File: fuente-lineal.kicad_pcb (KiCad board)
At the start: 2 copper layers, 100 x 74 mm, 34 parts, among them J1 Conn_01x03, J2 Conn_01x03, J3 Conn_01x01, J4 Conn_01x01, J5 Conn_01x01, J6 Conn_01x01, J7 Conn_01x01, J8 Conn_01x01, J9 Conn_01x02, U1 LM7805_TO220

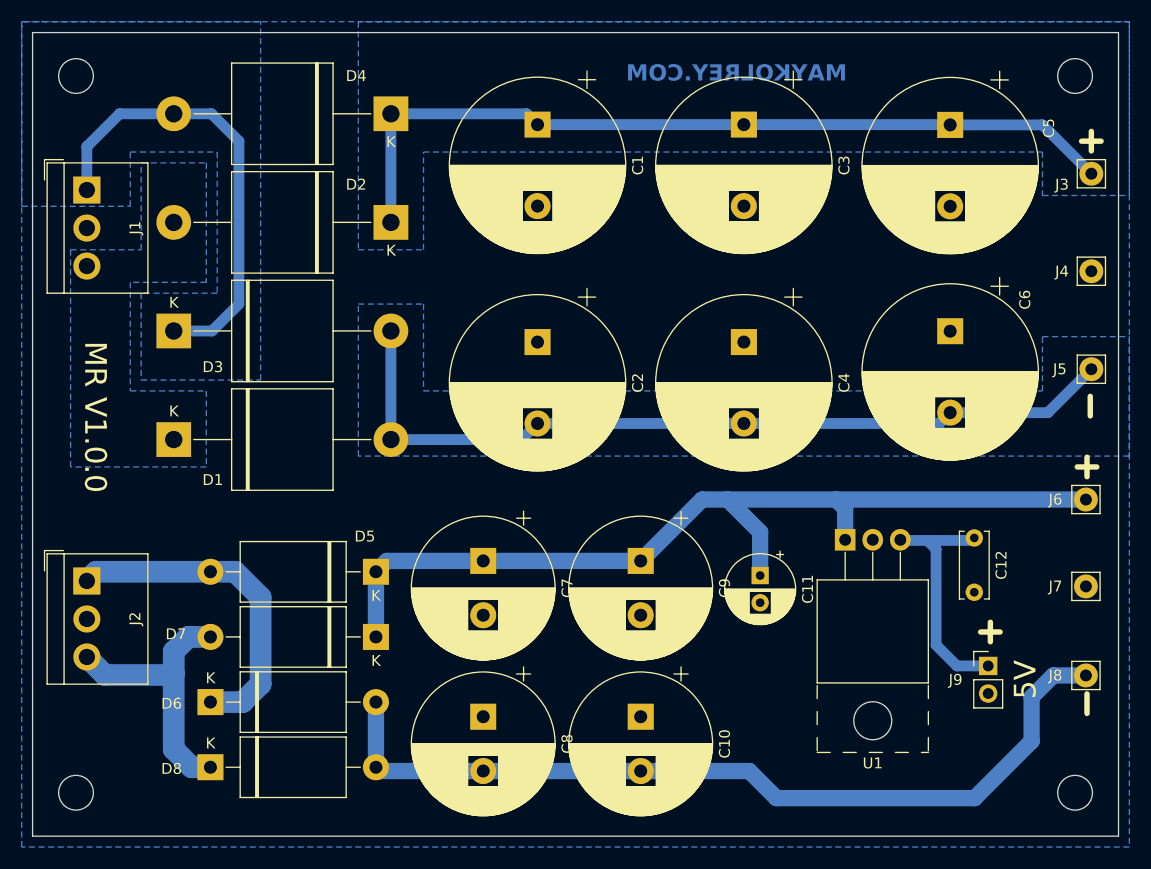
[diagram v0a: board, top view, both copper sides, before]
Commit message: completando version v1.1.0
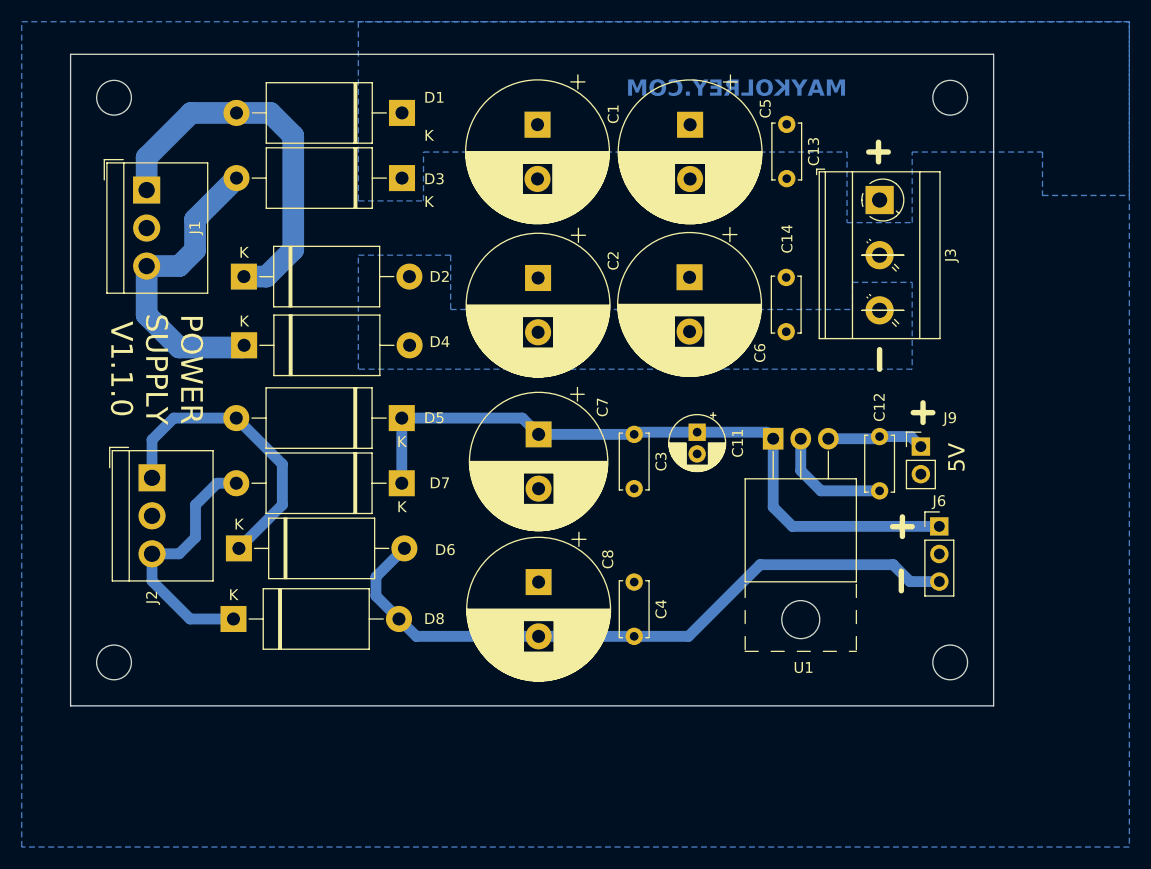
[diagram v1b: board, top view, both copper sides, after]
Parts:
- removed C10, C9: 2200uF, Capacitor_THT:CP_Radial_D13.0mm_P5.00mm
- removed J4, J5, J7, J8: Conn_01x01, Connector_Pin:Pin_D1.1mm_L8.5mm_W2.5mm_FlatFork
- added C13: 100nF, Capacitor_THT:C_Disc_D5.0mm_W2.5mm_P5.00mm, F.Cu at (164.4, 71.5)
- added C14: 100nF, Capacitor_THT:C_Disc_D5.0mm_W2.5mm_P5.00mm, F.Cu at (164.4, 85.5)
- C1, C2, C5, C6: footprint Capacitor_THT:CP_Radial_D16.0mm_P7.50mm -> Capacitor_THT:CP_Radial_D13.0mm_P5.00mm
- C11: value 0.33u -> 2.2uF; footprint Capacitor_THT:CP_Radial_D6.3mm_P2.50mm -> Capacitor_THT:CP_Radial_D5.0mm_P2.00mm
- C12: value C -> 100nF; footprint Capacitor_THT:C_Disc_D6.0mm_W2.5mm_P5.00mm -> Capacitor_THT:C_Disc_D5.0mm_W2.5mm_P5.00mm
- C3, C4: value 2200uF -> 100nF; footprint Capacitor_THT:CP_Radial_D16.0mm_P7.50mm -> Capacitor_THT:C_Disc_D5.0mm_W2.5mm_P5.00mm
- C7: footprint Capacitor_THT:CP_Radial_D13.0mm_P5.00mm -> Capacitor_THT:CP_Radial_D12.5mm_P5.00mm
- D1, D2, D3, D4: value 6A10 -> 1N5404; footprint Diode_THT:D_P600_R-6_P20.00mm_Horizontal -> Diode_THT:D_DO-27_P15.24mm_Horizontal
- J3: value Conn_01x01 -> Conn_01x03; footprint Connector_Pin:Pin_D1.1mm_L8.5mm_W2.5mm_FlatFork -> TerminalBlock_MetzConnect:TerminalBlock_MetzConnect_Type073_RT02603HBLU_1x03_P5.08mm_Horizontal
- J6: value Conn_01x01 -> Conn_01x03; footprint Connector_Pin:Pin_D1.1mm_L8.5mm_W2.5mm_FlatFork -> Connector_PinHeader_2.54mm:PinHeader_1x03_P2.54mm_Vertical
- moved D1 36.7 mm to (129.0, 70.4), turned to 180 degrees
- moved C3 30.3 mm to (150.4, 100.0)
- moved D3 25.3 mm to (129.0, 76.4), turned to 180 degrees
- moved D4 25.2 mm to (114.5, 91.8), turned to 0 degrees
- moved C6 24.5 mm to (155.5, 85.5)
- moved C4 24.3 mm to (150.4, 113.6)
- moved C5 24.0 mm to (155.6, 71.5)
- moved J9 21.1 mm to (176.8, 101.1)
- moved J3 19.6 mm to (173.0, 78.4), turned to -90 degrees
- moved H4 16.6 mm to (179.5, 121.0)
- moved D2 14.4 mm to (114.5, 85.5), turned to 0 degrees
- moved C11 14.4 mm to (156.2, 99.8)
- moved D6 14.4 mm to (114.0, 110.5)
- moved D5 14.4 mm to (129.0, 98.5)
- moved D7 14.4 mm to (129.0, 104.5)
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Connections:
- C3 pad 1: /Vop -> /Vo2p
- C4 pad 2: /Von -> /Vo2n
- D1 pad 1: /V2i -> /Vop
- D1 pad 2: /Von -> /V1i
- D2 pad 1: /Vop -> /V1i
- D2 pad 2: /V2i -> /Von
- D3 pad 1: /V1i -> /Vop
- D3 pad 2: /Von -> /V2i
- D4 pad 1: /Vop -> /V2i
- D4 pad 2: /V1i -> /Von
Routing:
- net /Von: track 77.2 -> 0.00 mm
- net /Vop: track 76.8 -> 0.00 mm
- net /V2i: track 0.00 -> 28.1 mm
- net /Vo2p: track 86.4 -> 63.5 mm
- net /Vo2n: track 79.6 -> 62.3 mm
- net /+5V: track 22.5 -> 8.99 mm
- net GND: track 0.00 -> 11.0 mm
- net /V1i: track 42.3 -> 35.1 mm
- net /V3i: track 30.6 -> 27.5 mm
- net /V4i: track 25.7 -> 23.7 mm
- removed copper zone on B.Cu, net /V1i
- removed copper zone on B.Cu, net /V2i
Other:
- board size 100 x 74 mm -> 85 x 60 mm
- board text added: "0"
- board text added: "0 mm"
- board text added: "0.01 mm"
- board text added: "0.02"
- board text added: "0.035 mm"
- board text added: "0.2000 mm / 0.2000 mm"
- board text added: "0.3000 mm"
- board text added: "1"
- board text added: "1.51 mm"
- board text added: "1.6000 mm"
- board text added: "2"
- board text added: "3.3"
- board text added: "4.5"
- board text added: "85.0000 mm x 60.0000 mm"
- board text added: "B.Cu"
- board text added: "B.Mask"
- board text added: "B.Paste"
- board text added: "B.Silkscreen"
- board text added: "BOARD CHARACTERISTICS"
- board text added: "Board Thickness:"
- board text added: "Board overall dimensions:"
- board text added: "Bottom Silk Screen"
- board text added: "Bottom Solder Mask"
- board text added: "Bottom Solder Paste"
- board text added: "Castellated pads:"
- board text added: "Color"
- board text added: "Copper Finish:"
- board text added: "Copper Layer Count:"
- board text added: "Dielectric 1"
- board text added: "Direct Printing"
- board text added: "Edge card connectors:"
- board text added: "Epsilon R"
- board text added: "F.Cu"
- board text added: "F.Mask"
- board text added: "F.Paste"
- board text added: "F.Silkscreen"
- board text added: "FR4"
- board text added: "FR4 natural"
- board text added: "Green"
- board text added: "HAL SnPb"
- board text added: "Impedance Control:"
- board text added: "Layer Name"
- board text added: "Liquid Ink"
- board text added: "Loss Tangent"
- board text added: "Material"
- board text added: "Min hole diameter:"
- board text added: "Min track/spacing:"
- board text added: "No"
- board text added: "POWER SUPPLY ${REVISION}"
- board text added: "Plated Board Edge:"
- board text added: "Thickness (mm)"
- board text added: "Top Silk Screen"
- board text added: "Top Solder Mask"
- board text added: "Top Solder Paste"
- board text added: "Type"
- board text added: "White"
- board text added: "copper"
- board text added: "core"
- board text removed: "MR ${REVISION}"
